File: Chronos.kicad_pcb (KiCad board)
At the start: 2 copper layers, 285 x 94.6 mm, 256 parts, among them Q1 NSS40301MZ4T1G, SW1 SW_PUSH, U1 ATMEGA32U2-AU, Y1 16MHz

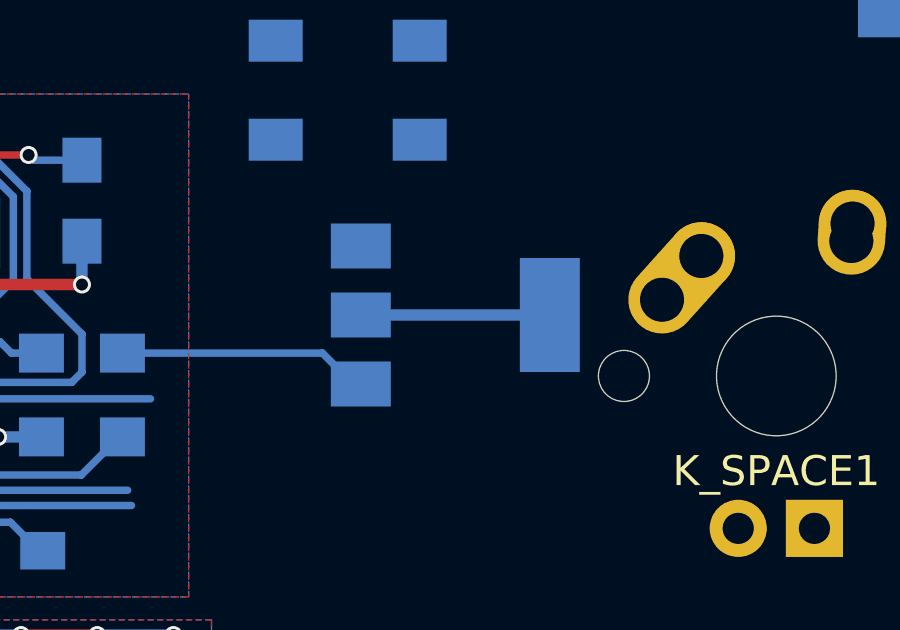
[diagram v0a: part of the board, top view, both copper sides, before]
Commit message: Change RGBLED pin
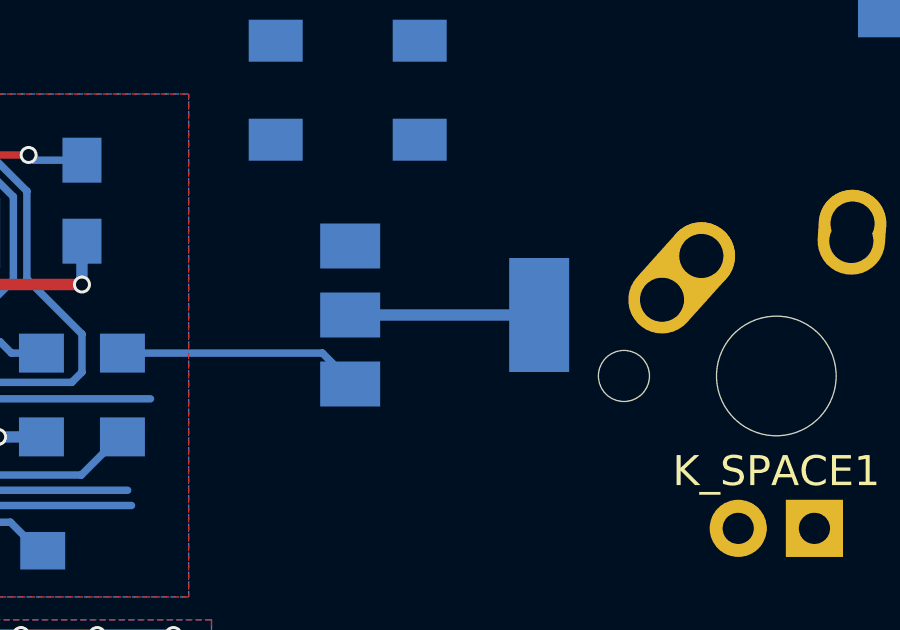
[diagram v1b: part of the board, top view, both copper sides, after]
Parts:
- moved Q1 0.36 mm to (167.5, 131.3)
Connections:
- U1 pad 23: Net-(U1-Pad23) -> RGBLED
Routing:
- net RGBLED: track 0.00 -> 7.01 mm
- net Net-(U1-Pad23): track 7.01 -> 0.00 mm
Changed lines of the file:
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@@
 (kicad_pcb (version 4) (host pcbnew 4.0.6)
   (general
-    (links 641)
-    (no_connects 456)
+    (links 642)
+    (no_connects 457)
     (area 0 0 0 0)
     (thickness 1.6)
@@
     (zones 0)
     (modules 256)
-    (nets 249)
+    (nets 248)
   )
   (page A3)
@@
   (net 235 "Net-(U1-Pad20)")
   (net 236 "Net-(U1-Pad22)")
-  (net 237 "Net-(U1-Pad23)")
-  (net 238 "Net-(U1-Pad25)")
-  (net 239 "Net-(U1-Pad26)")
-  (net 240 "Net-(USB1-Pad2)")
-  (net 241 "Net-(K_SHIFT2-Pad2)")
-  (net 242 "Net-(K_SHIFT2-Pad1)")
-  (net 243 "Net-(K_SHIFT2-Pad3)")
-  (net 244 "Net-(K_SHIFT2-Pad4)")
-  (net 245 "Net-(K_CAPS2-Pad2)")
-  (net 246 "Net-(K_CAPS2-Pad1)")
-  (net 247 "Net-(K_CAPS2-Pad3)")
-  (net 248 "Net-(K_CAPS2-Pad4)")
+  (net 237 "Net-(U1-Pad25)")
+  (net 238 "Net-(U1-Pad26)")
+  (net 239 "Net-(USB1-Pad2)")
+  (net 240 "Net-(K_SHIFT2-Pad2)")
+  (net 241 "Net-(K_SHIFT2-Pad1)")
+  (net 242 "Net-(K_SHIFT2-Pad3)")
+  (net 243 "Net-(K_SHIFT2-Pad4)")
+  (net 244 "Net-(K_CAPS2-Pad2)")
+  (net 245 "Net-(K_CAPS2-Pad1)")
+  (net 246 "Net-(K_CAPS2-Pad3)")
+  (net 247 "Net-(K_CAPS2-Pad4)")
   (net_class Default "This is the default net class."
     (clearance 0.2)
@@
     (add_net "Net-(U1-Pad20)")
     (add_net "Net-(U1-Pad22)")
-    (add_net "Net-(U1-Pad23)")
     (add_net "Net-(U1-Pad25)")
     (add_net "Net-(U1-Pad26)")
@@
   )
   (module TO_SOT_Packages_SMD:SOT-223-3_TabPin2 (layer B.Cu)
-    (at 167.894 131.318)
+    (at 167.538 131.318)
     (descr "module CMS SOT223 4 pins")
     (tags "CMS SOT")
@@
       (net 236 "Net-(U1-Pad22)"))
     (pad 23 smd rect (at 4.25 2) (size 1.6 0.55) (layers B.Cu B.Paste B.Mask)
-      (net 237 "Net-(U1-Pad23)"))
+      (net 207 RGBLED))
     (pad 24 smd rect (at 4.25 2.8) (size 1.6 0.55) (layers B.Cu B.Paste B.Mask)
       (net 199 "Net-(R1-Pad2)"))
     (pad 25 smd rect (at 2.8 4.25 270) (size 1.6 0.55) (layers B.Cu B.Paste B.Mask)
-      (net 238 "Net-(U1-Pad25)"))
+      (net 237 "Net-(U1-Pad25)"))
     (pad 26 smd rect (at 2 4.25 270) (size 1.6 0.55) (layers B.Cu B.Paste B.Mask)
-      (net 239 "Net-(U1-Pad26)"))
+      (net 238 "Net-(U1-Pad26)"))
     (pad 27 smd rect (at 1.2 4.25 270) (size 1.6 0.55) (layers B.Cu B.Paste B.Mask)
       (net 4 "Net-(C3-Pad1)"))
@@
       (net 2 GND))
     (pad 2 smd rect (at 4.5 -0.8 270) (size 2.25 0.5) (layers B.Cu B.Paste B.Mask)
-      (net 240 "Net-(USB1-Pad2)"))
+      (net 239 "Net-(USB1-Pad2)"))
     (pad 3 smd rect (at 4.5 0 270) (size 2.25 0.5) (layers B.Cu B.Paste B.Mask)
       (net 201 DP))
@@
     (fp_line (start -11.90625 9.525) (end -11.90625 -9.525) (layer Dwgs.User) (width 0.15))
     (pad 2 thru_hole oval (at 2.5 -4.5 86.0548) (size 2.831378 2.25) (drill 1.47 (offset 0.290689 0)) (layers *.Cu *.Mask)
-      (net 241 "Net-(K_SHIFT2-Pad2)"))
+      (net 240 "Net-(K_SHIFT2-Pad2)"))
     (pad 2 thru_hole circle (at 2.54 -5.08) (size 2.25 2.25) (drill 1.47) (layers *.Cu *.Mask)
-      (net 241 "Net-(K_SHIFT2-Pad2)"))
+      (net 240 "Net-(K_SHIFT2-Pad2)"))
     (pad 1 thru_hole oval (at -3.81 -2.54 48.09963212) (size 4.211556 2.25) (drill 1.47 (offset 0.980778 0)) (layers *.Cu *.Mask)
-      (net 242 "Net-(K_SHIFT2-Pad1)"))
+      (net 241 "Net-(K_SHIFT2-Pad1)"))
     (pad "" np_thru_hole circle (at 0 0) (size 3.9878 3.9878) (drill 3.9878) (layers *.Cu *.Mask))
     (pad 1 thru_hole circle (at -2.5 -4) (size 2.25 2.25) (drill 1.47) (layers *.Cu *.Mask)
-      (net 242 "Net-(K_SHIFT2-Pad1)"))
+      (net 241 "Net-(K_SHIFT2-Pad1)"))
     (pad 3 thru_hole circle (at -1.27 5.08) (size 1.905 1.905) (drill 1.04) (layers *.Cu *.Mask)
-      (net 243 "Net-(K_SHIFT2-Pad3)"))
+      (net 242 "Net-(K_SHIFT2-Pad3)"))
     (pad 4 thru_hole rect (at 1.27 5.08) (size 1.905 1.905) (drill 1.04) (layers *.Cu *.Mask)
-      (net 244 "Net-(K_SHIFT2-Pad4)"))
+      (net 243 "Net-(K_SHIFT2-Pad4)"))
     (pad "" np_thru_hole circle (at -5.08 0 48.0996) (size 1.7018 1.7018) (drill 1.7018) (layers *.Cu *.Mask))
     (pad "" np_thru_hole circle (at 5.08 0 48.0996) (size 1.7018 1.7018) (drill 1.7018) (layers *.Cu *.Mask))
@@
     (fp_line (start -11.90625 9.525) (end -11.90625 -9.525) (layer Dwgs.User) (width 0.15))
     (pad 2 thru_hole oval (at 2.5 -4.5 86.0548) (size 2.831378 2.25) (drill 1.47 (offset 0.290689 0)) (layers *.Cu *.Mask)
-      (net 245 "Net-(K_CAPS2-Pad2)"))
+      (net 244 "Net-(K_CAPS2-Pad2)"))
     (pad 2 thru_hole circle (at 2.54 -5.08) (size 2.25 2.25) (drill 1.47) (layers *.Cu *.Mask)
-      (net 245 "Net-(K_CAPS2-Pad2)"))
+      (net 244 "Net-(K_CAPS2-Pad2)"))
     (pad 1 thru_hole oval (at -3.81 -2.54 48.09963212) (size 4.211556 2.25) (drill 1.47 (offset 0.980778 0)) (layers *.Cu *.Mask)
-      (net 246 "Net-(K_CAPS2-Pad1)"))
+      (net 245 "Net-(K_CAPS2-Pad1)"))
     (pad "" np_thru_hole circle (at 0 0) (size 3.9878 3.9878) (drill 3.9878) (layers *.Cu *.Mask))
     (pad 1 thru_hole circle (at -2.5 -4) (size 2.25 2.25) (drill 1.47) (layers *.Cu *.Mask)
-      (net 246 "Net-(K_CAPS2-Pad1)"))
+      (net 245 "Net-(K_CAPS2-Pad1)"))
     (pad 3 thru_hole circle (at -1.27 5.08) (size 1.905 1.905) (drill 1.04) (layers *.Cu *.Mask)
-      (net 247 "Net-(K_CAPS2-Pad3)"))
+      (net 246 "Net-(K_CAPS2-Pad3)"))
     (pad 4 thru_hole rect (at 1.27 5.08) (size 1.905 1.905) (drill 1.04) (layers *.Cu *.Mask)
-      (net 248 "Net-(K_CAPS2-Pad4)"))
+      (net 247 "Net-(K_CAPS2-Pad4)"))
     (pad "" np_thru_hole circle (at -5.08 0 48.0996) (size 1.7018 1.7018) (drill 1.7018) (layers *.Cu *.Mask))
     (pad "" np_thru_hole circle (at 5.08 0 48.0996) (size 1.7018 1.7018) (drill 1.7018) (layers *.Cu *.Mask))
@@
   (segment (start 153.844 126.158) (end 153.67 125.984) (width 0.25) (layer B.Cu) (net 205))
   (via (at 153.67 125.984) (size 0.6) (drill 0.4) (layers F.Cu B.Cu) (net 205))
+  (segment (start 152.36909 134.112) (end 157.734 134.112) (width 0.25) (layer B.Cu) (net 207))
+  (segment (start 150.8535 133.81) (end 152.06709 133.81) (width 0.25) (layer B.Cu) (net 207))
+  (segment (start 152.06709 133.81) (end 152.36909 134.112) (width 0.25) (layer B.Cu) (net 207))
   (segment (start 139.192 126.01914) (end 139.192 122.936) (width 0.25) (layer B.Cu) (net 221))
   (segment (start 139.936 127.492) (end 139.936 126.76314) (width 0.25) (layer B.Cu) (net 221))
@@
   (segment (start 152.456501 133.563001) (end 155.108001 133.563001) (width 0.25) (layer B.Cu) (net 236))
   (segment (start 155.108001 133.563001) (end 155.448 133.223002) (width 0.25) (layer B.Cu) (net 236))
-  (segment (start 152.36909 134.112) (end 157.734 134.112) (width 0.25) (layer B.Cu) (net 237))
-  (segment (start 150.8535 133.81) (end 152.06709 133.81) (width 0.25) (layer B.Cu) (net 237))
-  (segment (start 152.06709 133.81) (end 152.36909 134.112) (width 0.25) (layer B.Cu) (net 237))
-  (segment (start 151.0285 137.16) (end 149.9285 136.06) (width 0.25) (layer B.Cu) (net 238))
-  (segment (start 156.972 137.16) (end 151.0285 137.16) (width 0.25) (layer B.Cu) (net 238))
-  (segment (start 149.9285 136.06) (end 149.4035 136.06) (width 0.25) (layer B.Cu) (net 238))
-  (segment (start 149.1615 137.668) (end 157.10041 137.668) (width 0.25) (layer B.Cu) (net 239))
-  (segment (start 148.6035 136.06) (end 148.6035 137.11) (width 0.25) (layer B.Cu) (net 239))
-  (segment (start 148.6035 137.11) (end 149.1615 137.668) (width 0.25) (layer B.Cu) (net 239))
+  (segment (start 151.0285 137.16) (end 149.9285 136.06) (width 0.25) (layer B.Cu) (net 237))
+  (segment (start 156.972 137.16) (end 151.0285 137.16) (width 0.25) (layer B.Cu) (net 237))
+  (segment (start 149.9285 136.06) (end 149.4035 136.06) (width 0.25) (layer B.Cu) (net 237))
+  (segment (start 149.1615 137.668) (end 157.10041 137.668) (width 0.25) (layer B.Cu) (net 238))
+  (segment (start 148.6035 136.06) (end 148.6035 137.11) (width 0.25) (layer B.Cu) (net 238))
+  (segment (start 148.6035 137.11) (end 149.1615 137.668) (width 0.25) (layer B.Cu) (net 238))
   (zone (net 2) (net_name GND) (layer B.Cu) (hatch edge 0.508)
     (connect_pads (clearance 0.254))
